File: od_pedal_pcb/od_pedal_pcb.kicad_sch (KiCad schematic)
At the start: 30 parts, among them J1 JST_VDD, J3 JST_IN, J4 JST_OUT, U1 TL072

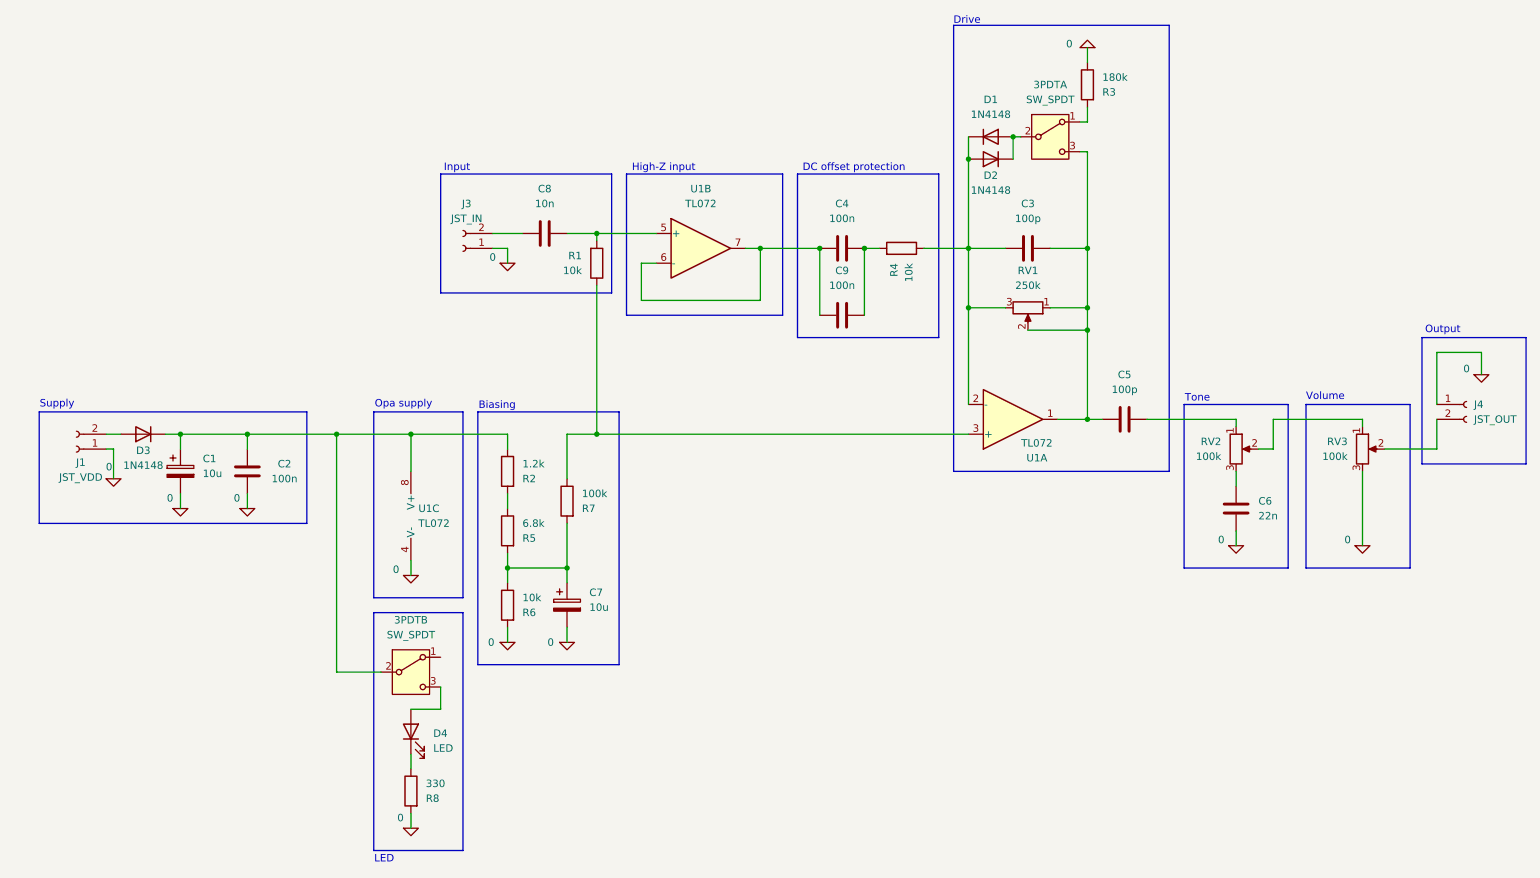
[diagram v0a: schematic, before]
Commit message: feat: changes to bypass
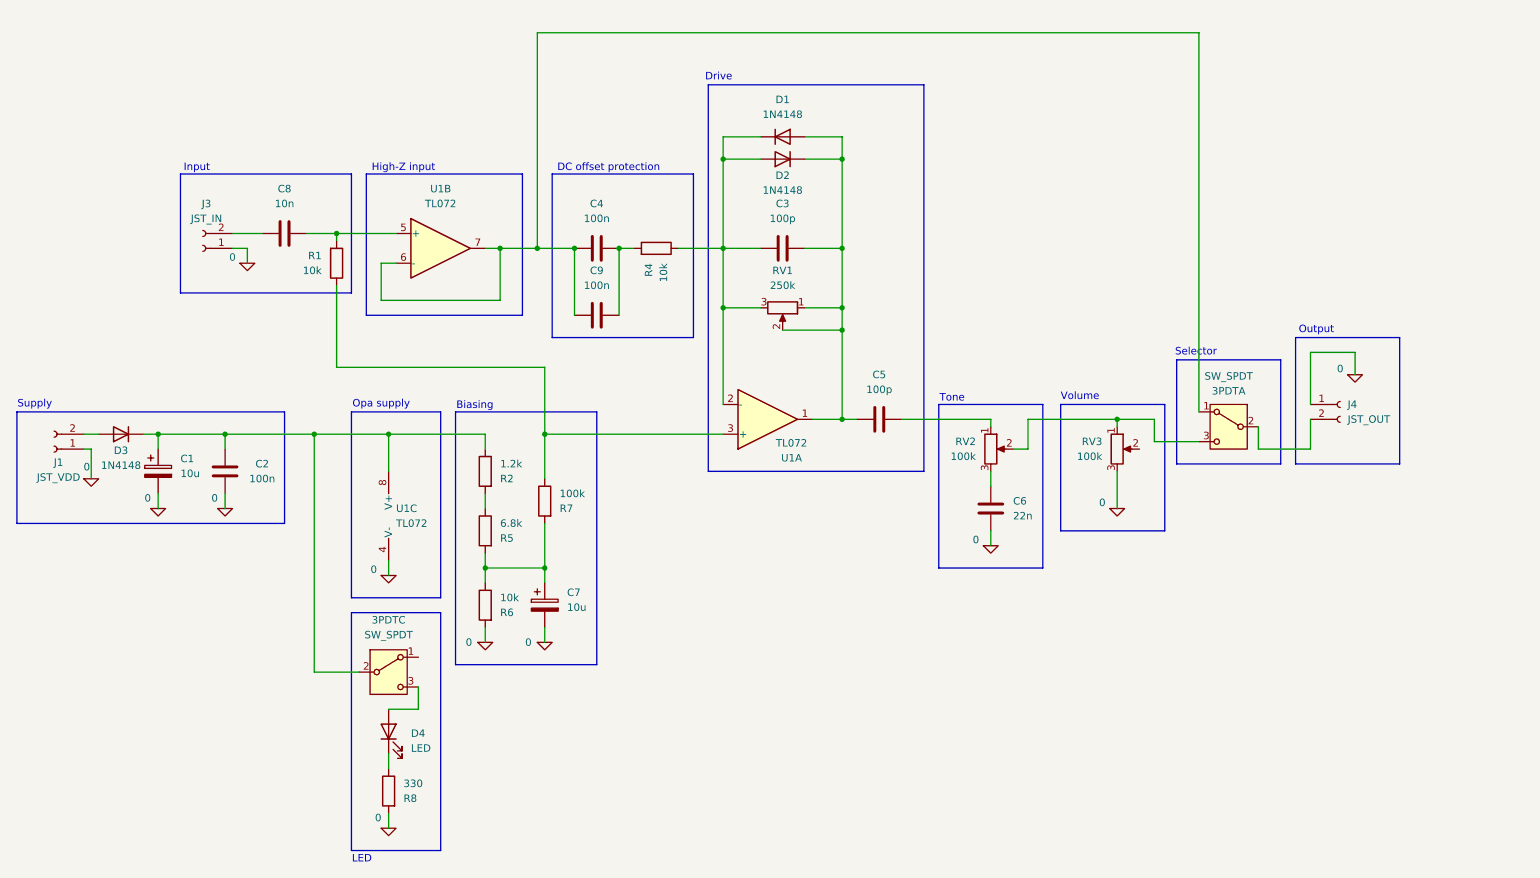
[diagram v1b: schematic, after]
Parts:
- removed R3: 180k, Resistor_THT:R_Axial_DIN0207_L6.3mm_D2.5mm_P10.16mm_Horizontal, symbol Device:R
- renumbered 3PDTB to 3PDTC
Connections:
- net at RV2.2, RV3.1: now also 3PDTA.3 (C)
- net at J4.2 (Pin_2): now also 3PDTA.2 (B); no longer RV3.2
- net at C3.2, C5.1, RV1.1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: now also D1.2 (A), D2.1 (K); no longer 3PDTA.3 (C)
- net at 3PDTA.1 (A): now also C4.1, C9.1, U1.6 (-), U1.7
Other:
- note added: "Selector"
- moved on the sheet: 3PDTC, C1, C2, C3, C4, C5, C6, C7, C8, C9, D1, D2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
